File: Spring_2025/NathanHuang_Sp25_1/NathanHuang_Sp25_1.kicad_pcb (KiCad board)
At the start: 2 copper layers, 122.3 x 92.8 mm, 19 parts, among them J1 Barrel_Jack, M1 Motor_Servo, M2 Motor_Servo, M3 Motor_Servo, M4 Motor_Servo, M5 Motor_Servo, M6 Motor_Servo, M7 Stepper_Motor_bipolar, SW1 SW_SPST, SW2 SW_SPST, U1 ESP32-WROOM-32, U2 LM2596_BUCK_CONVERTER, U3 Pololu_Breakout_A4988

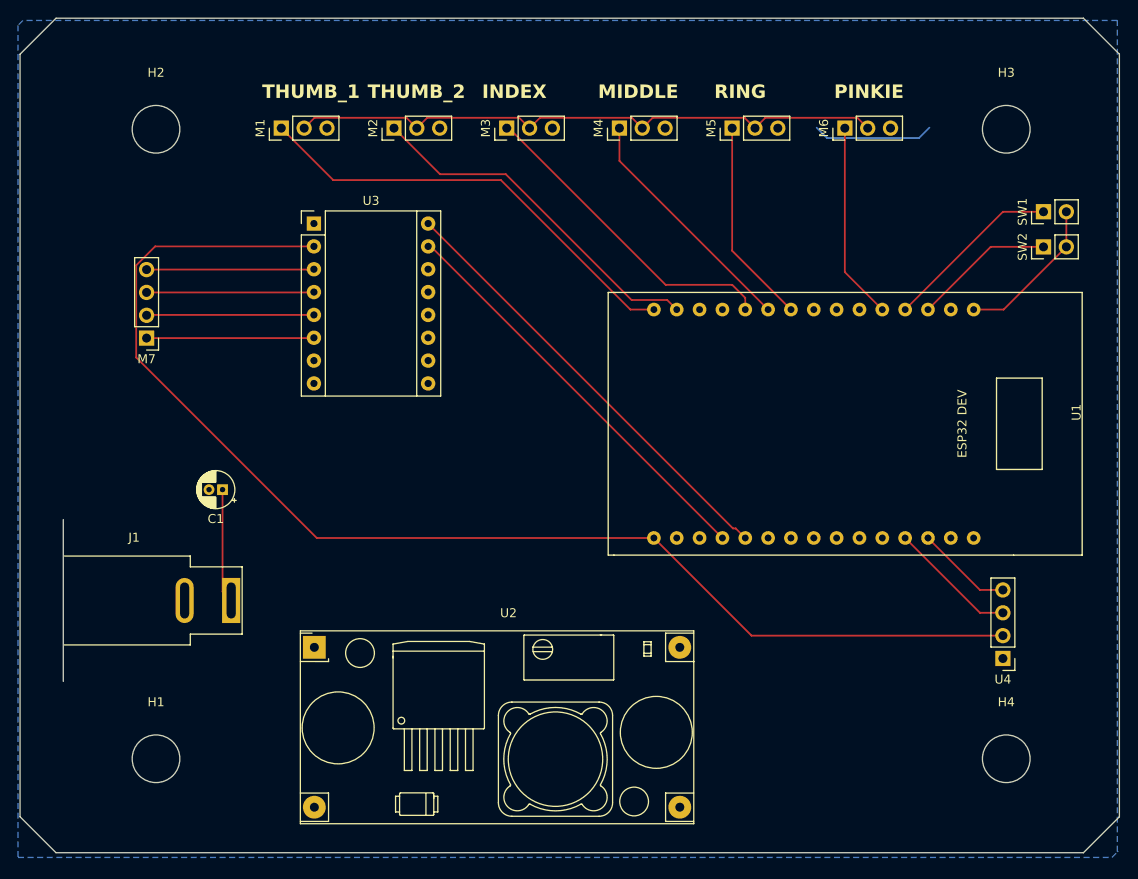
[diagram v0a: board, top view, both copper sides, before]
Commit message: Gerbers ready
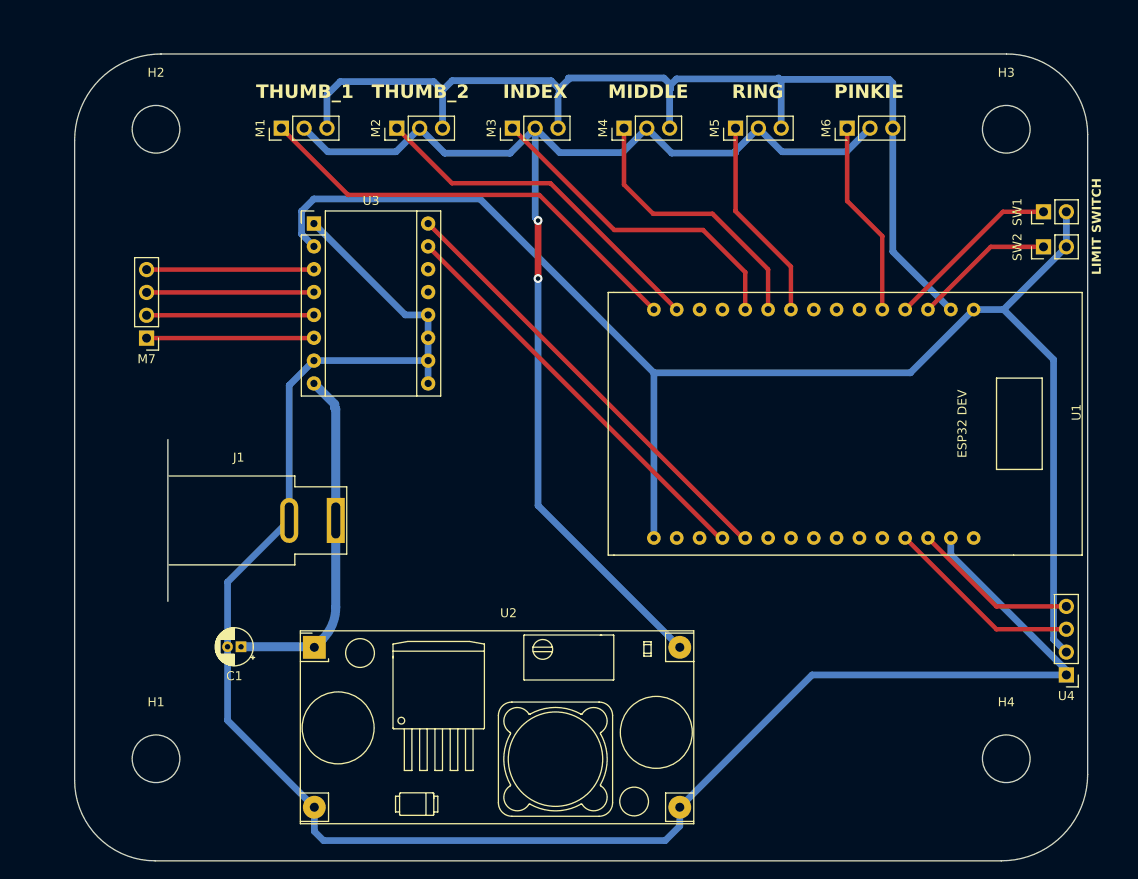
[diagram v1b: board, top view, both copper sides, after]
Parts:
- moved C1 17.6 mm to (94.1, 124.7)
- moved J1 14.6 mm to (104.7, 110.7)
- moved U4 7.29 mm to (185.9, 127.8)
- moved M3 0.63 mm to (124.3, 67.0)
- moved M4 0.50 mm to (136.7, 67.0)
- moved M5 0.38 mm to (149.1, 67.0)
- moved M2 0.32 mm to (111.4, 67.0)
- moved M6 0.25 mm to (161.5, 67.0)
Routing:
- net GND: track 13.5 -> 327.7 mm
- net 7.2V: track 67.4 -> 138.7 mm, vias 0 -> 2
- net +12V: track 12.7 -> 39.3 mm
- net +3V3: track 157.2 -> 167.1 mm
- net /DT: track 10.7 -> 18.5 mm
- net /CW: track 14.3 -> 22.1 mm
- net /MIDDLE: track 27.0 -> 30.7 mm
- net /INDEX: track 35.6 -> 36.7 mm
- removed copper zone on B.Cu, net GND
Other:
- board size 122.3 x 92.8 mm -> 112.7 x 89.7 mm
- board text added: "LIMIT SWITCH"
